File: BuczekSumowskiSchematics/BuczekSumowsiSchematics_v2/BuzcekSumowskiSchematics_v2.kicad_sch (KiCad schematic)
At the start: 13 parts

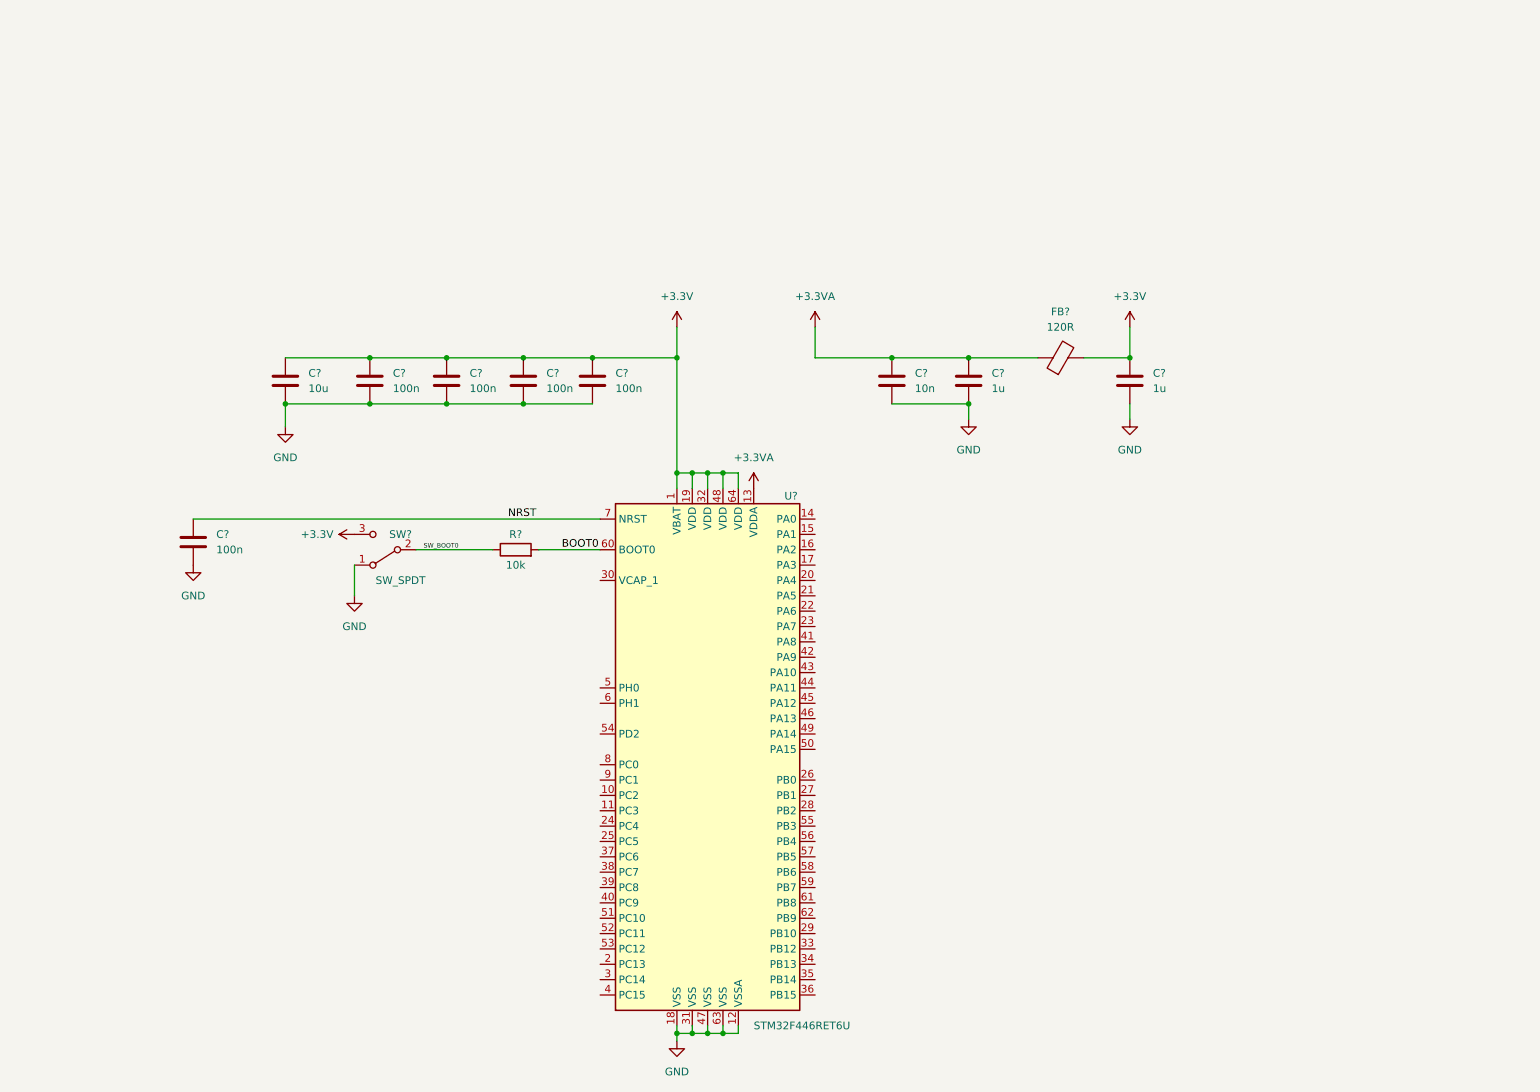
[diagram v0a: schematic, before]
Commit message: schemtics progress
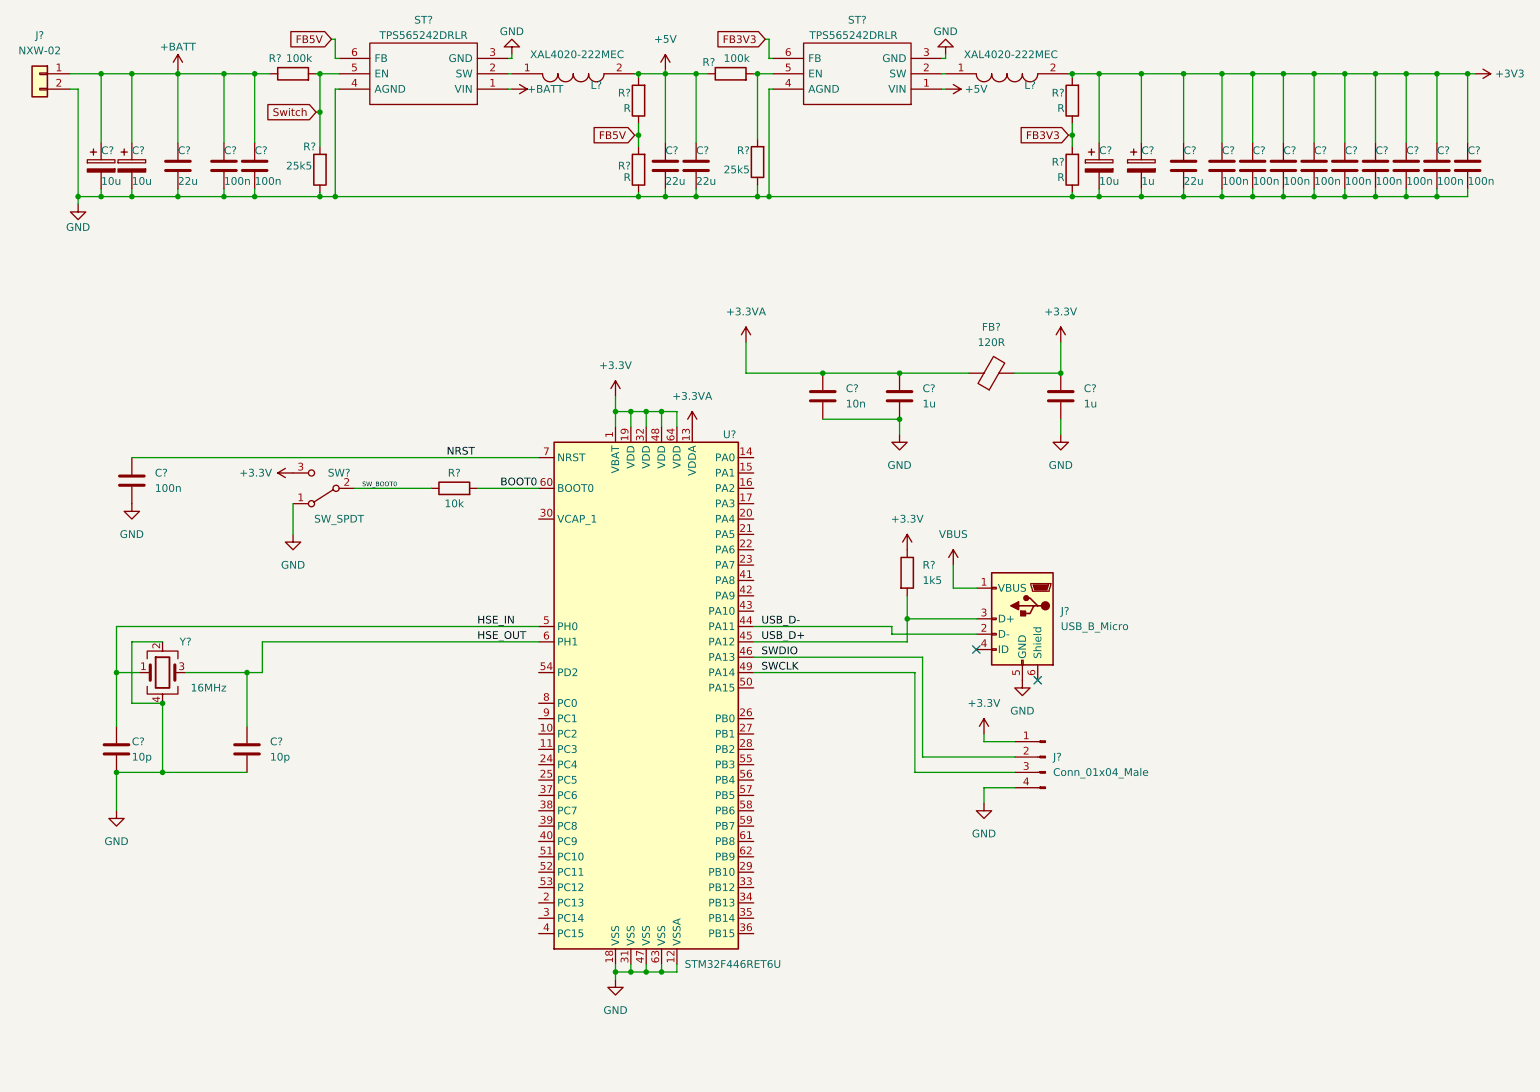
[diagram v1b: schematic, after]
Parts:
- removed C?: 10u, symbol Device:C
- removed C? (x4): 100n, symbol Device:C
- added C? (x2): 10p, symbol Device:C
- added C? (x11): 100n, Capacitor_SMD:C_0805_2012Metric_Pad1.18x1.45mm_HandSolder, symbol Device:C
- added C? (x4): 22u, Capacitor_SMD:C_0805_2012Metric_Pad1.18x1.45mm_HandSolder, symbol Device:C
- added C? (x3): 10u, Capacitor_Tantalum_SMD:CP_EIA-3216-18_Kemet-A_Pad1.58x1.35mm_HandSolder, symbol Device:C_Polarized
- added C?: 1u, Capacitor_Tantalum_SMD:CP_EIA-3216-18_Kemet-A_Pad1.58x1.35mm_HandSolder, symbol Device:C_Polarized
- added J?: USB_B_Micro, symbol Connector:USB_B_Micro
- added J?: NXW-02, Connector_Molex:Molex_Micro-Latch_53253-0270_1x02_P2.00mm_Vertical, symbol Connector_Generic:Conn_01x02
- added J?: Conn_01x04_Male, symbol Connector:Conn_01x04_Male
- added L? (x2): XAL4020-222MEC, Inductor_SMD:L_Coilcraft_XxL4040, symbol SamacSys_Parts:XAL4020-222MEC
- added R? (x4): R, Resistor_SMD:R_0805_2012Metric_Pad1.20x1.40mm_HandSolder, symbol Device:R
- added R?: 1k5, symbol Device:R
- added R? (x2): 100k, Resistor_SMD:R_0805_2012Metric_Pad1.20x1.40mm_HandSolder, symbol Device:R
- added R? (x2): 25k5, Resistor_SMD:R_0805_2012Metric_Pad1.20x1.40mm_HandSolder, symbol Device:R
- added ST? (x2): TPS565242DRLR, Package_TO_SOT_SMD:SOT-563, symbol SamacSys_Parts:TPS565242DRLR
- added Y?: 16MHz, symbol Device:Crystal_GND24
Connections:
- net +3.3V: now also J?.1 (Pin_1), R?.1
- net GND: now also C?.2, C?.2, C?.2, C?.2, C?.2, C?.2, C?.2, C?.2, C?.2, C?.2, C?.2, C?.2, C?.2, C?.2, C?.2, C?.2, C?.2, C?.2, C?.2, C?.2, C?.2, J?.2 (Pin_2), J?.4 (Pin_4), J?.5 (GND), R?.1, R?.1, R?.1, R?.1, ST?.3 (GND), ST?.3 (GND), ST?.4 (AGND), ST?.4 (AGND), Y?.2, Y?.4
- net USB_D-: now reaches U?.44 (PA11)
- net USB_D-: now also J?.2 (D-)
- net USB_D+: now reaches U?.45 (PA12)
- net USB_D+: now also J?.3 (D+), R?.2
- net SWDIO: now reaches U?.46 (PA13)
- net SWDIO: now also J?.2 (Pin_2)
- net SWCLK: now reaches U?.49 (PA14)
- net SWCLK: now also J?.3 (Pin_3)
- net HSE_IN: now reaches U?.5 (PH0)
- net HSE_IN: now also C?.1, Y?.1
- net HSE_OUT: now reaches U?.6 (PH1)
- net HSE_OUT: now also C?.1, Y?.3
- new net: L?.1, ST?.2 (SW) (x2)
- new net: R?.2, R?.2, ST?.5 (EN)
- new net +3V3: C?.1, C?.1, C?.1, C?.1, C?.1, C?.1, C?.1, C?.1, C?.1, C?.1, C?.1, C?.1, L?.2, R?.2
- new net +5V: C?.1, C?.1, L?.2, R?.1, R?.2, ST?.1 (VIN)
- new net +BATT: C?.1, C?.1, C?.1, C?.1, C?.1, J?.1 (Pin_1), R?.1, ST?.1 (VIN)
- new net FB3V3: R?.1, R?.2, ST?.6 (FB)
- new net FB5V: R?.1, R?.2, ST?.6 (FB)
- new net Switch: R?.2, R?.2, ST?.5 (EN)
- new net VBUS: J?.1 (VBUS)
- no-connect marks 0 -> 2
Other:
- moved on the sheet: C?, FB?, R?, SW?, U?
